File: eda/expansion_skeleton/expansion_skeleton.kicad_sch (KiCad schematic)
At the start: 4 parts

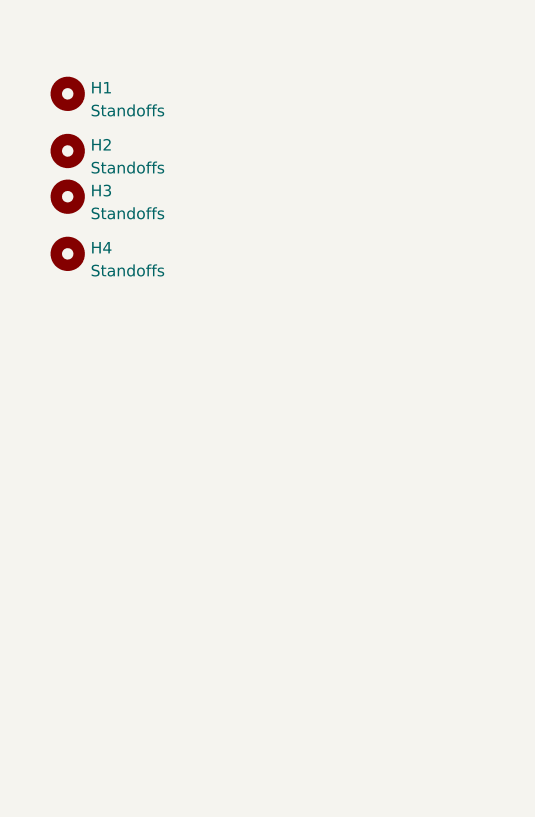
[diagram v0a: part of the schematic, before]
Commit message: Branch of uart to v1
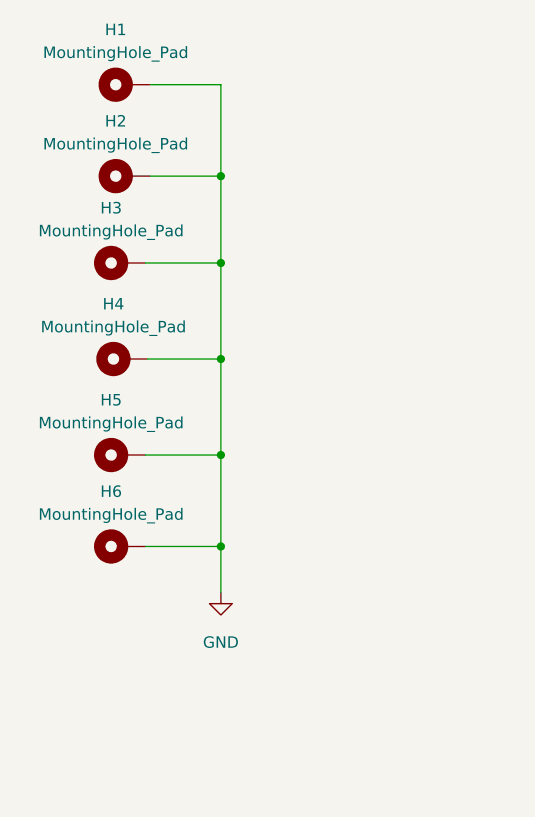
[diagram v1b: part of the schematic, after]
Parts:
- removed H1, H2, H3, H4: Standoffs, MountingHole:MountingHole_2.5mm, symbol Mechanical:MountingHole
- added H1, H2, H3, H4, H5, H6: MountingHole_Pad, MountingHole:MountingHole_2.5mm_Pad_Via, symbol Mechanical:MountingHole_Pad
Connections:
- new net GND: H1.1, H2.1, H3.1, H4.1, H5.1, H6.1
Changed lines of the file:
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@@
 (kicad_sch (version 20230121) (generator eeschema)
   (paper "A4")
-  (symbol (lib_id "Mechanical:MountingHole") (at 21.59 34.29 0) (unit 1)
-    (in_bom yes) (on_board yes) (dnp no) (fields_autoplaced)
-    (property "Reference" "H3" (at 24.13 33.655 0)
-      (effects (font (size 1.27 1.27)) (justify left))
-    )
-    (property "Value" "Standoffs" (at 24.13 36.195 0)
-      (effects (font (size 1.27 1.27)) (justify left))
-    )
-    (property "Footprint" "MountingHole:MountingHole_2.5mm" (at 21.59 34.29 0)
-      (effects (font (size 1.27 1.27)) hide)
-    )
-    (property "Datasheet" "~" (at 21.59 34.29 0)
-      (effects (font (size 1.27 1.27)) hide)
-    )
+  (junction (at 38.608 41.656) (diameter 0) (color 0 0 0 0)
+  )
+  (junction (at 38.608 62.992) (diameter 0) (color 0 0 0 0)
+  )
+  (junction (at 38.608 52.324) (diameter 0) (color 0 0 0 0)
+  )
+  (junction (at 38.608 32.004) (diameter 0) (color 0 0 0 0)
+  )
+  (junction (at 38.608 73.152) (diameter 0) (color 0 0 0 0)
+  )
+  (wire (pts (xy 30.734 21.844) (xy 38.608 21.844))
+    (stroke (width 0) (type default))
+  )
+  (wire (pts (xy 38.608 73.152) (xy 38.608 78.232))
+    (stroke (width 0) (type default))
+  )
+  (wire (pts (xy 38.608 52.324) (xy 38.608 62.992))
+    (stroke (width 0) (type default))
+  )
+  (wire (pts (xy 30.734 32.004) (xy 38.608 32.004))
+    (stroke (width 0) (type default))
+  )
+  (wire (pts (xy 38.608 21.844) (xy 38.608 32.004))
+    (stroke (width 0) (type default))
+  )
+  (wire (pts (xy 30.48 52.324) (xy 38.608 52.324))
+    (stroke (width 0) (type default))
+  )
+  (wire (pts (xy 38.608 32.004) (xy 38.608 41.656))
+    (stroke (width 0) (type default))
+  )
+  (wire (pts (xy 38.608 62.992) (xy 38.608 73.152))
+    (stroke (width 0) (type default))
+  )
+  (wire (pts (xy 38.608 41.656) (xy 38.608 52.324))
+    (stroke (width 0) (type default))
+  )
+  (wire (pts (xy 30.226 62.992) (xy 38.608 62.992))
+    (stroke (width 0) (type default))
+  )
+  (wire (pts (xy 30.226 73.152) (xy 38.608 73.152))
+    (stroke (width 0) (type default))
+  )
+  (wire (pts (xy 30.226 41.656) (xy 38.608 41.656))
+    (stroke (width 0) (type default))
+  )
+  (symbol (lib_id "Mechanical:MountingHole_Pad") (at 28.194 21.844 90) (unit 1)
+    (in_bom yes) (on_board yes) (dnp no) (fields_autoplaced)
+    (property "Reference" "H1" (at 26.924 15.748 90)
+      (effects (font (size 1.27 1.27)))
+    )
+    (property "Value" "MountingHole_Pad" (at 26.924 18.288 90)
+      (effects (font (size 1.27 1.27)))
+    )
+    (property "Footprint" "MountingHole:MountingHole_2.5mm_Pad_Via" (at 28.194 21.844 0)
+      (effects (font (size 1.27 1.27)) hide)
+    )
+    (property "Datasheet" "~" (at 28.194 21.844 0)
+      (effects (font (size 1.27 1.27)) hide)
+    )
+    (pin "1")
+    (instances
+      (project "expansion_skeleton"
+        (path "/f65326c0-118f-43ae-8d7d-86cc11609fcf"
+          (reference "H1") (unit 1)
+        )
+      )
+    )
+  )
+  (symbol (lib_id "Mechanical:MountingHole_Pad") (at 28.194 32.004 90) (unit 1)
+    (in_bom yes) (on_board yes) (dnp no) (fields_autoplaced)
+    (property "Reference" "H2" (at 26.924 25.908 90)
+      (effects (font (size 1.27 1.27)))
+    )
+    (property "Value" "MountingHole_Pad" (at 26.924 28.448 90)
+      (effects (font (size 1.27 1.27)))
+    )
+    (property "Footprint" "MountingHole:MountingHole_2.5mm_Pad_Via" (at 28.194 32.004 0)
+      (effects (font (size 1.27 1.27)) hide)
+    )
+    (property "Datasheet" "~" (at 28.194 32.004 0)
+      (effects (font (size 1.27 1.27)) hide)
+    )
+    (pin "1")
+    (instances
+      (project "expansion_skeleton"
+        (path "/f65326c0-118f-43ae-8d7d-86cc11609fcf"
+          (reference "H2") (unit 1)
+        )
+      )
+    )
+  )
+  (symbol (lib_id "Mechanical:MountingHole_Pad") (at 27.686 73.152 90) (unit 1)
+    (in_bom yes) (on_board yes) (dnp no) (fields_autoplaced)
+    (property "Reference" "H6" (at 26.416 67.056 90)
+      (effects (font (size 1.27 1.27)))
+    )
+    (property "Value" "MountingHole_Pad" (at 26.416 69.596 90)
+      (effects (font (size 1.27 1.27)))
+    )
+    (property "Footprint" "MountingHole:MountingHole_2.5mm_Pad_Via" (at 27.686 73.152 0)
+      (effects (font (size 1.27 1.27)) hide)
+    )
+    (property "Datasheet" "~" (at 27.686 73.152 0)
+      (effects (font (size 1.27 1.27)) hide)
+    )
+    (pin "1")
+    (instances
+      (project "expansion_skeleton"
+        (path "/f65326c0-118f-43ae-8d7d-86cc11609fcf"
+          (reference "H6") (unit 1)
+        )
+      )
+    )
+  )
+  (symbol (lib_id "Mechanical:MountingHole_Pad") (at 27.686 62.992 90) (unit 1)
+    (in_bom yes) (on_board yes) (dnp no) (fields_autoplaced)
+    (property "Reference" "H5" (at 26.416 56.896 90)
+      (effects (font (size 1.27 1.27)))
+    )
+    (property "Value" "MountingHole_Pad" (at 26.416 59.436 90)
+      (effects (font (size 1.27 1.27)))
+    )
+    (property "Footprint" "MountingHole:MountingHole_2.5mm_Pad_Via" (at 27.686 62.992 0)
+      (effects (font (size 1.27 1.27)) hide)
+    )
+    (property "Datasheet" "~" (at 27.686 62.992 0)
+      (effects (font (size 1.27 1.27)) hide)
+    )
+    (pin "1")
+    (instances
+      (project "expansion_skeleton"
+        (path "/f65326c0-118f-43ae-8d7d-86cc11609fcf"
+          (reference "H5") (unit 1)
+        )
+      )
+    )
+  )
+  (symbol (lib_id "Mechanical:MountingHole_Pad") (at 27.686 41.656 90) (unit 1)
+    (in_bom yes) (on_board yes) (dnp no) (fields_autoplaced)
+    (property "Reference" "H3" (at 26.416 35.56 90)
+      (effects (font (size 1.27 1.27)))
+    )
+    (property "Value" "MountingHole_Pad" (at 26.416 38.1 90)
+      (effects (font (size 1.27 1.27)))
+    )
+    (property "Footprint" "MountingHole:MountingHole_2.5mm_Pad_Via" (at 27.686 41.656 0)
+      (effects (font (size 1.27 1.27)) hide)
+    )
+    (property "Datasheet" "~" (at 27.686 41.656 0)
+      (effects (font (size 1.27 1.27)) hide)
+    )
+    (pin "1")
     (instances
       (project "expansion_skeleton"
@@
     )
   )
-  (symbol (lib_id "Mechanical:MountingHole") (at 21.59 40.64 0) (unit 1)
-    (in_bom yes) (on_board yes) (dnp no) (fields_autoplaced)
-    (property "Reference" "H4" (at 24.13 40.005 0)
-      (effects (font (size 1.27 1.27)) (justify left))
-    )
-    (property "Value" "Standoffs" (at 24.13 42.545 0)
-      (effects (font (size 1.27 1.27)) (justify left))
-    )
-    (property "Footprint" "MountingHole:MountingHole_2.5mm" (at 21.59 40.64 0)
-      (effects (font (size 1.27 1.27)) hide)
-    )
-    (property "Datasheet" "~" (at 21.59 40.64 0)
-      (effects (font (size 1.27 1.27)) hide)
-    )
+  (symbol (lib_id "Mechanical:MountingHole_Pad") (at 27.94 52.324 90) (unit 1)
+    (in_bom yes) (on_board yes) (dnp no) (fields_autoplaced)
+    (property "Reference" "H4" (at 26.67 46.228 90)
+      (effects (font (size 1.27 1.27)))
+    )
+    (property "Value" "MountingHole_Pad" (at 26.67 48.768 90)
+      (effects (font (size 1.27 1.27)))
+    )
+    (property "Footprint" "MountingHole:MountingHole_2.5mm_Pad_Via" (at 27.94 52.324 0)
+      (effects (font (size 1.27 1.27)) hide)
+    )
+    (property "Datasheet" "~" (at 27.94 52.324 0)
+      (effects (font (size 1.27 1.27)) hide)
+    )
+    (pin "1")
     (instances
       (project "expansion_skeleton"
@@
     )
   )
-  (symbol (lib_id "Mechanical:MountingHole") (at 21.59 22.86 0) (unit 1)
-    (in_bom yes) (on_board yes) (dnp no) (fields_autoplaced)
-    (property "Reference" "H1" (at 24.13 22.225 0)
-      (effects (font (size 1.27 1.27)) (justify left))
-    )
-    (property "Value" "Standoffs" (at 24.13 24.765 0)
-      (effects (font (size 1.27 1.27)) (justify left))
-    )
-    (property "Footprint" "MountingHole:MountingHole_2.5mm" (at 21.59 22.86 0)
-      (effects (font (size 1.27 1.27)) hide)
-    )
-    (property "Datasheet" "~" (at 21.59 22.86 0)
-      (effects (font (size 1.27 1.27)) hide)
-    )
-    (instances
-      (project "expansion_skeleton"
-        (path "/f65326c0-118f-43ae-8d7d-86cc11609fcf"
-          (reference "H1") (unit 1)
-        )
-      )
-    )
-  )
-  (symbol (lib_id "Mechanical:MountingHole") (at 21.59 29.21 0) (unit 1)
-    (in_bom yes) (on_board yes) (dnp no) (fields_autoplaced)
-    (property "Reference" "H2" (at 24.13 28.575 0)
-      (effects (font (size 1.27 1.27)) (justify left))
-    )
-    (property "Value" "Standoffs" (at 24.13 31.115 0)
-      (effects (font (size 1.27 1.27)) (justify left))
-    )
-    (property "Footprint" "MountingHole:MountingHole_2.5mm" (at 21.59 29.21 0)
-      (effects (font (size 1.27 1.27)) hide)
-    )
-    (property "Datasheet" "~" (at 21.59 29.21 0)
-      (effects (font (size 1.27 1.27)) hide)
-    )
-    (instances
-      (project "expansion_skeleton"
-        (path "/f65326c0-118f-43ae-8d7d-86cc11609fcf"
-          (reference "H2") (unit 1)
-        )
-      )
+  (symbol (lib_id "power:GND") (at 38.608 78.232 0) (unit 1)
+    (in_bom yes) (on_board yes) (dnp no) (fields_autoplaced)
+    (property "Reference" "#PWR01" (at 38.608 84.582 0)
+      (effects (font (size 1.27 1.27)) hide)
+    )
+    (property "Value" "GND" (at 38.608 83.82 0)
+      (effects (font (size 1.27 1.27)))
+    )
+    (property "Footprint" "" (at 38.608 78.232 0)
+      (effects (font (size 1.27 1.27)) hide)
+    )
+    (property "Datasheet" "" (at 38.608 78.232 0)
+      (effects (font (size 1.27 1.27)) hide)
+    )
+    (pin "1")
+    (instances
+      (project "expansion_skeleton"
+        (path "/f65326c0-118f-43ae-8d7d-86cc11609fcf"
+          (reference "#PWR01") (unit 1)
+        )
+      )
